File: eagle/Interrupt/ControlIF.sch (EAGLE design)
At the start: 8 parts

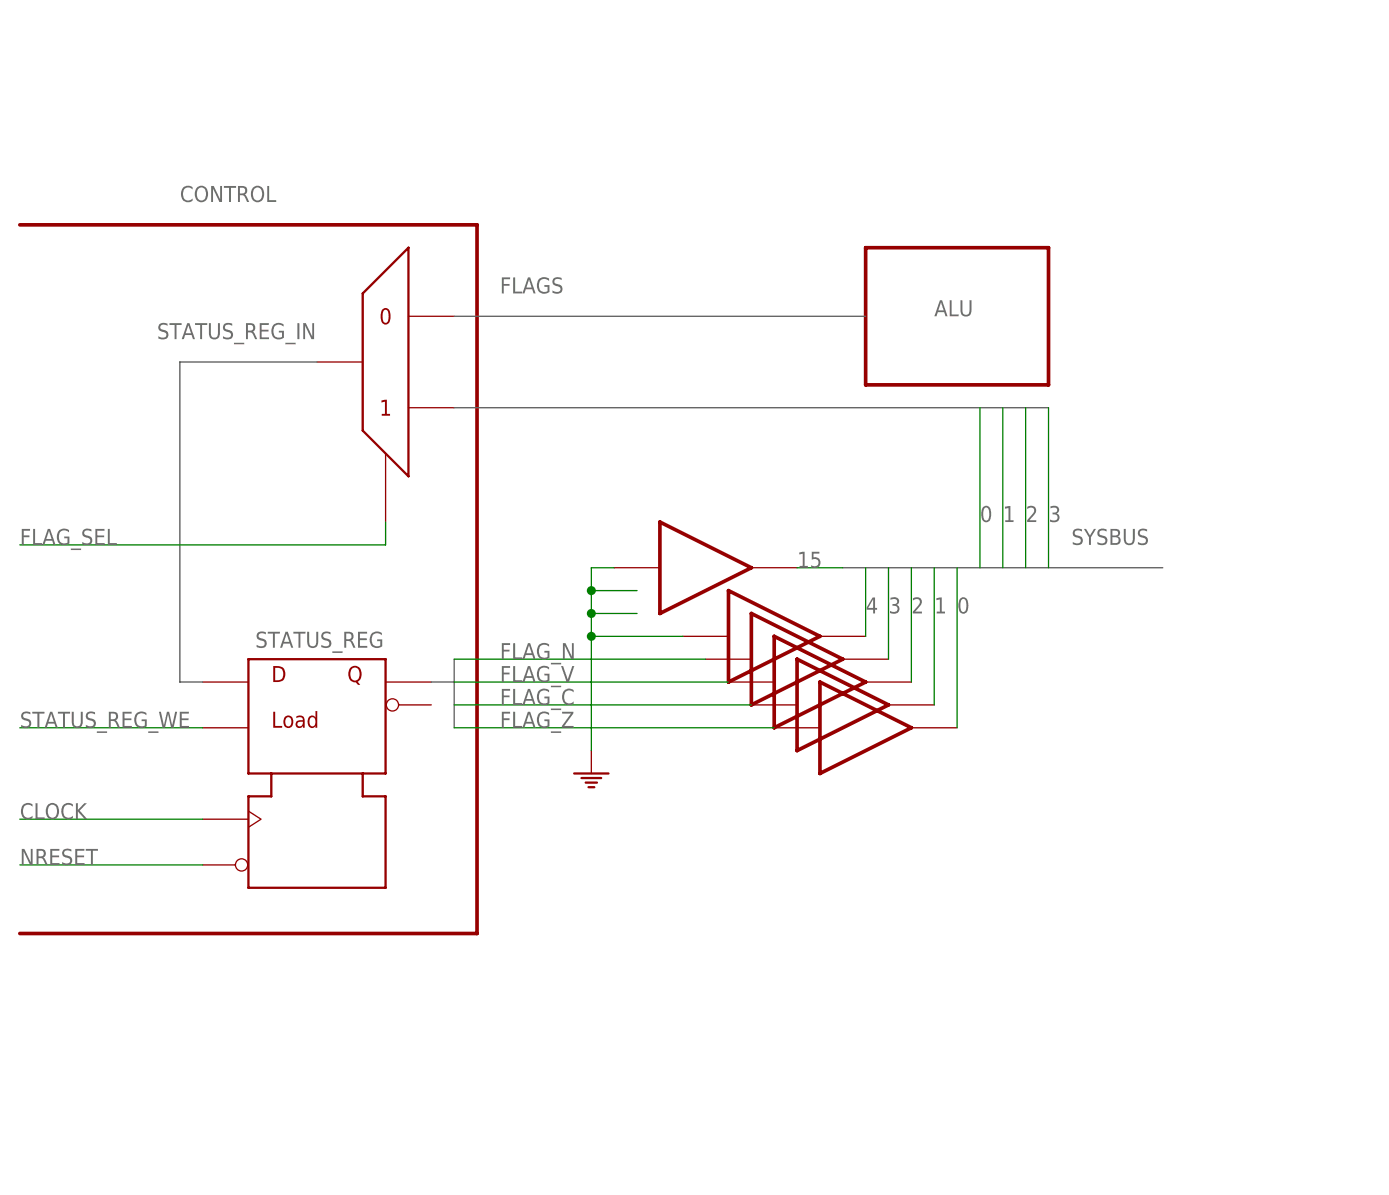
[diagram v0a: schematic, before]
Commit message: schmatic update
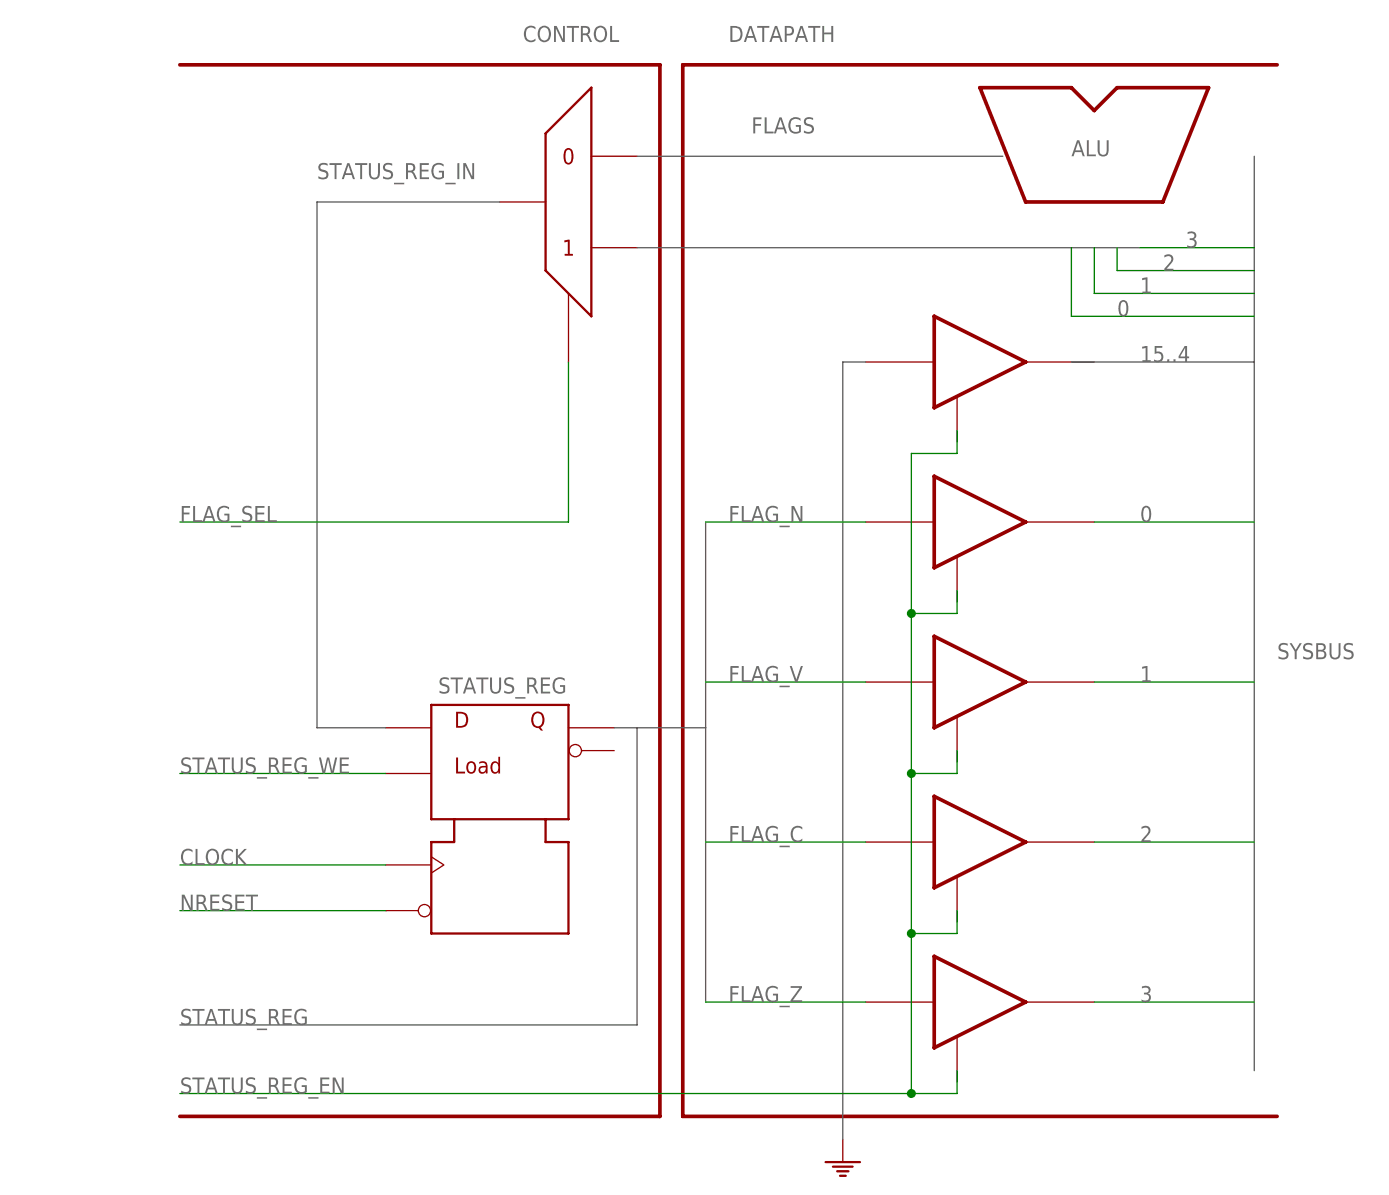
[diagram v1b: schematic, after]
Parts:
- removed BUFFER_0, BUFFER_1, BUFFER_15, BUFFER_2, BUFFER_3, BUFFER_4: BUFFER, c035u:BUFFER
- added TRISBUF_1, TRISBUF_2, TRISBUF_3, TRISBUF_4, TRISBUF_5: TRISBUF, c035u:TRISBUF
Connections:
- removed net 15: BUFFER_15.O
- removed net 4: BUFFER_4.O
- removed net FLAG_N: BUFFER_3.I
- removed net FLAG_V: BUFFER_2.I
- removed net PE: BUFFER_15.I, BUFFER_4.I
- net 0: now also TRISBUF_4.O; no longer BUFFER_0.O
- net 1: now also TRISBUF_3.O; no longer BUFFER_1.O
- net 2: now also TRISBUF_2.O; no longer BUFFER_2.O
- net 3: now also TRISBUF_1.O; no longer BUFFER_3.O
- net FLAG_C: now also TRISBUF_2.I; no longer BUFFER_1.I
- net FLAG_Z: now also TRISBUF_1.I; no longer BUFFER_0.I
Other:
- note added: "DATAPATH"
- moved on the sheet: STATUS_REG
